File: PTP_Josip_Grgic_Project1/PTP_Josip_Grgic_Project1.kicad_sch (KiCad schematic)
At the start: 24 parts, among them U1 NE555P, U2 LM2574N-5

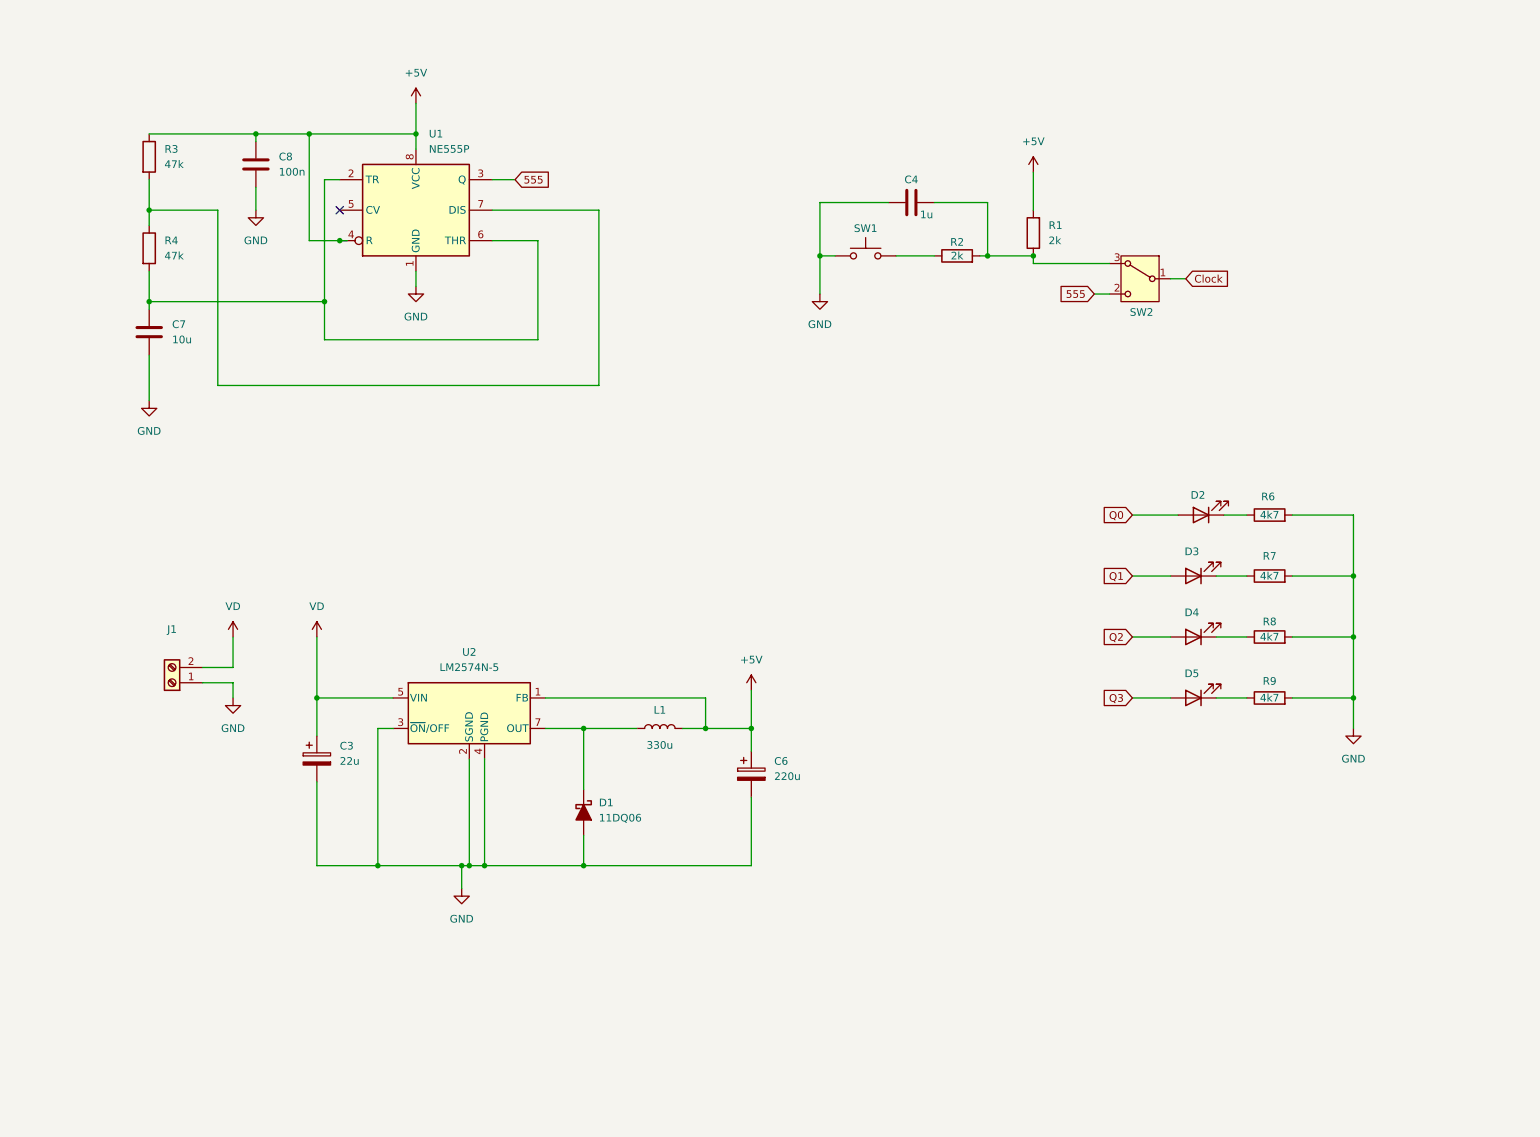
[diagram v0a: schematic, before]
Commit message: project1_lv3
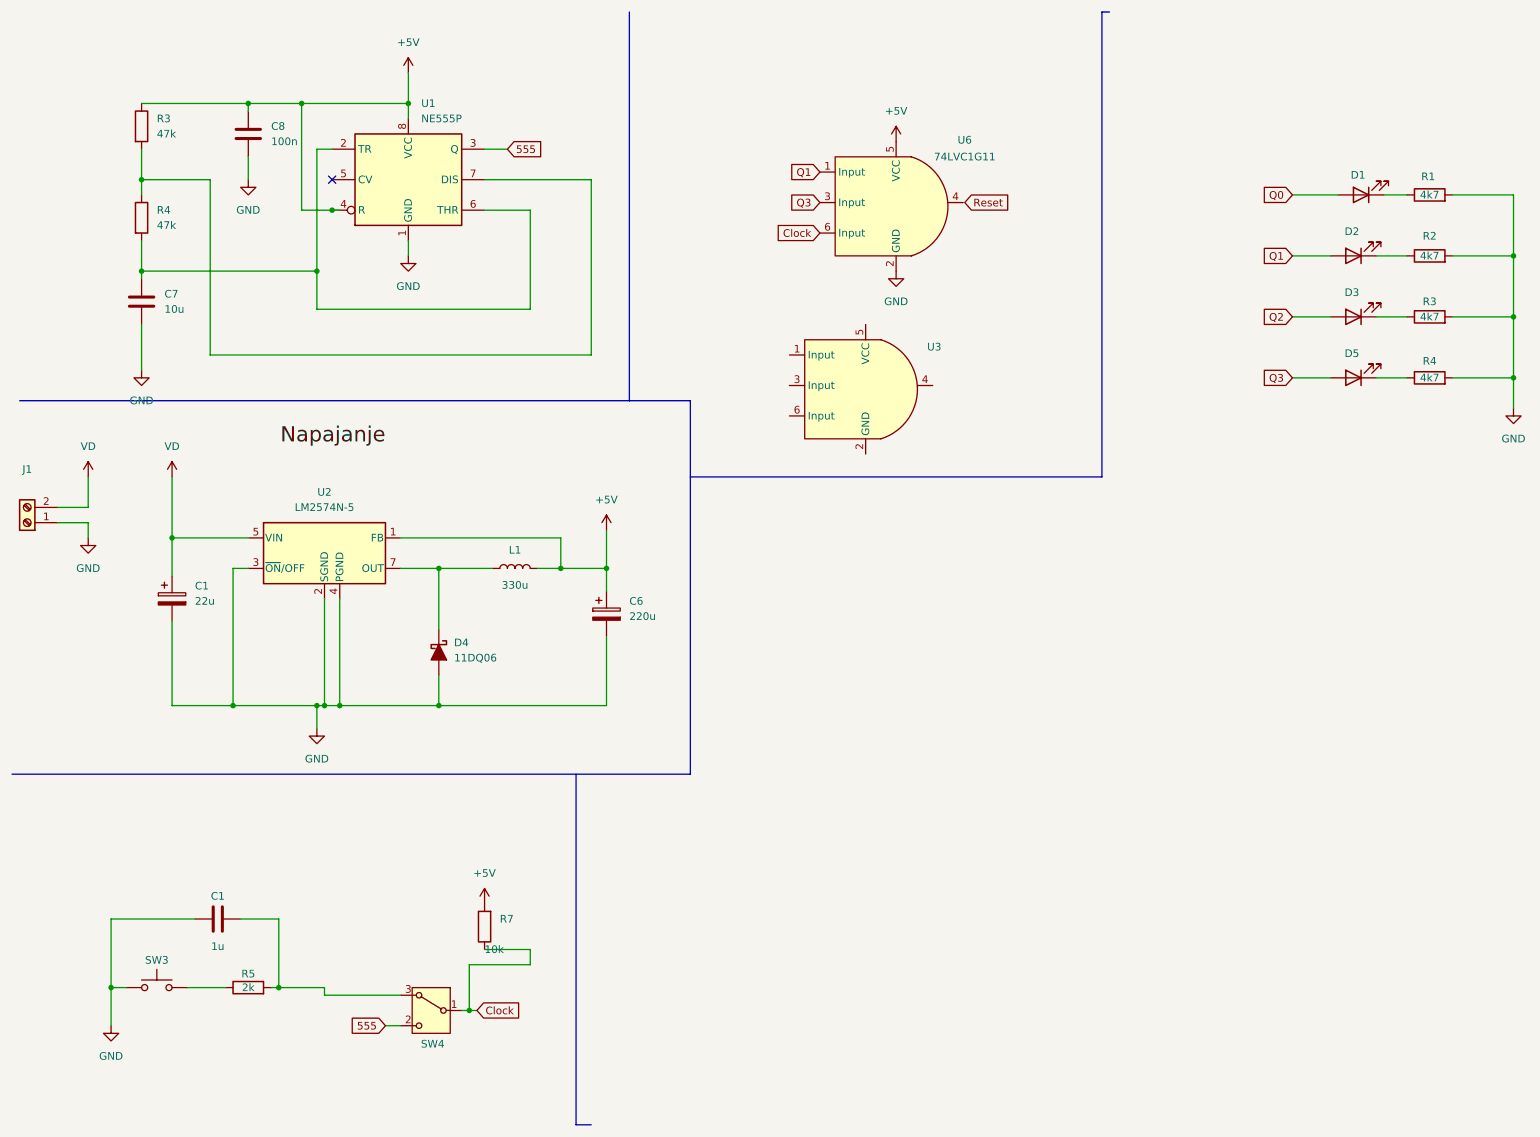
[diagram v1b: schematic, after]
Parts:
- removed C4: 1u, symbol Device:C
- removed R1, R2: 2k, symbol Device:R
- removed SW1: ~, symbol Switch:SW_Push
- removed SW2: ~, symbol Switch:SW_SPDT
- added C1: 1u, symbol Device:C
- added R5: 2k, symbol Device:R
- added R7: 10k, symbol Device:R
- added SW3: ~, symbol Switch:SW_Push
- added SW4: ~, symbol Switch:SW_SPDT
- added U3: ~, symbol SN74LVC1G11:SM74LVC1G11
- added U6: 74LVC1G11, symbol SN74LVC1G11:SM74LVC1G11
- renumbered C3 to C1, D2 to D1, D3 to D2, D4 to D3, D1 to D4, R6 to R1, R7 to R2, R8 to R3, R9 to R4
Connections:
- net +5V: now also R7.2, U6.5 (VCC)
- net 555: now also SW4.2 (C)
- net Clock: now also R7.1, SW4.1 (B), U6.6 (Input)
- net GND: now also C1.1, SW3.1, U6.2 (GND)
- net Q1: now also U6.1 (Input)
- net Q3: now also U6.3 (Input)
- new net: R5.1, SW3.2
- new net: C1.2, R5.2, SW4.3 (A)
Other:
- moved on the sheet: C1, C6, C7, C8, D1, D2, D3, D4, D5, J1, L1, R1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
